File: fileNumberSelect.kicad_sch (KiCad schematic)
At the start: 13 parts, among them U17 74AHC138, U19 74AHCT244, U20 74AHCT244, U21 74AHCT244, U22 74AHCT244, U23 74AHCT244

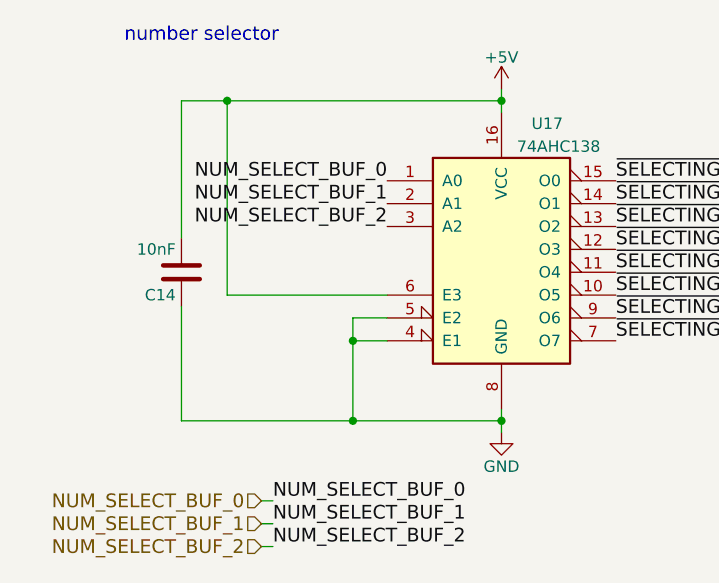
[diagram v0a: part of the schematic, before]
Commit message: bit of cleaning after last commit
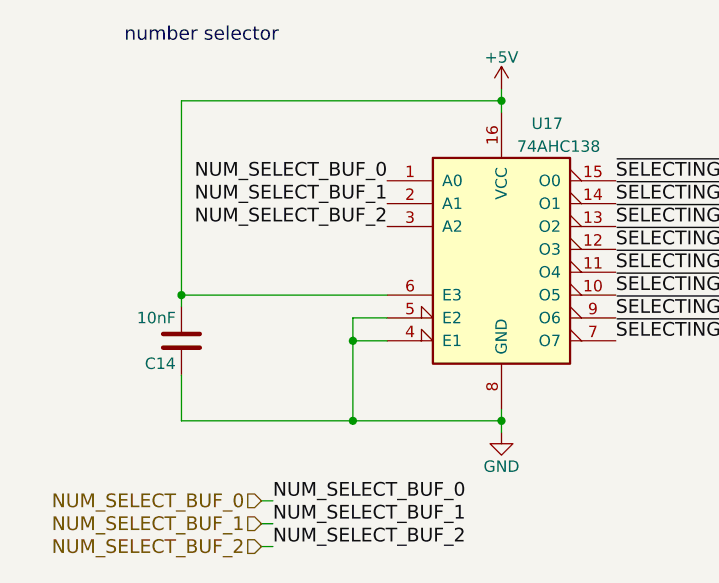
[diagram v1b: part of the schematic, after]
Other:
- moved on the sheet: C14
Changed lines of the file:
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@@
   (junction (at 62.23 24.13) (diameter 0) (color 0 0 0 0)
   )
+  (junction (at 26.67 45.72) (diameter 0) (color 0 0 0 0)
+  )
   (junction (at 238.76 149.86) (diameter 0) (color 0 0 0 0)
   )
@@
   (junction (at 220.98 22.86) (diameter 0) (color 0 0 0 0)
   )
-  (junction (at 31.75 24.13) (diameter 0) (color 0 0 0 0)
-  )
   (junction (at 218.44 25.4) (diameter 0) (color 0 0 0 0)
   )
@@
     (stroke (width 0) (type default) (color 0 0 0 0))
   )
-  (wire (pts (xy 31.75 24.13) (xy 31.75 45.72))
-    (stroke (width 0) (type default) (color 0 0 0 0))
-  )
   (wire (pts (xy 137.16 171.45) (xy 139.7 171.45))
     (stroke (width 0) (type default) (color 0 0 0 0))
@@
     (stroke (width 0) (type default) (color 0 0 0 0))
   )
-  (wire (pts (xy 31.75 24.13) (xy 26.67 24.13))
+  (wire (pts (xy 26.67 24.13) (xy 62.23 24.13))
     (stroke (width 0) (type default) (color 0 0 0 0))
   )
@@
     (stroke (width 0) (type default) (color 0 0 0 0))
   )
-  (wire (pts (xy 26.67 46.99) (xy 26.67 59.69))
+  (wire (pts (xy 26.67 54.61) (xy 26.67 59.69))
     (stroke (width 0) (type default) (color 0 0 0 0))
   )
@@
     (stroke (width 0) (type default) (color 0 0 0 0))
   )
-  (wire (pts (xy 26.67 24.13) (xy 26.67 39.37))
+  (wire (pts (xy 26.67 24.13) (xy 26.67 45.72))
     (stroke (width 0) (type default) (color 0 0 0 0))
   )
@@
     (stroke (width 0) (type default) (color 0 0 0 0))
   )
+  (wire (pts (xy 26.67 45.72) (xy 26.67 46.99))
+    (stroke (width 0) (type default) (color 0 0 0 0))
+  )
   (wire (pts (xy 43.18 151.13) (xy 44.45 151.13))
     (stroke (width 0) (type default) (color 0 0 0 0))
@@
     (stroke (width 0) (type default) (color 0 0 0 0))
   )
-  (wire (pts (xy 62.23 24.13) (xy 31.75 24.13))
-    (stroke (width 0) (type default) (color 0 0 0 0))
-  )
-  (wire (pts (xy 49.53 45.72) (xy 31.75 45.72))
+  (wire (pts (xy 26.67 45.72) (xy 49.53 45.72))
     (stroke (width 0) (type default) (color 0 0 0 0))
   )
@@
     (pin "1")
   )
-  (symbol (lib_id "Device:C") (at 26.67 43.18 180) (unit 1)
+  (symbol (lib_id "Device:C") (at 26.67 50.8 180) (unit 1)
     (in_bom yes) (on_board yes)
-    (property "Reference" "C14" (id 0) (at 26.035 45.72 0)
+    (property "Reference" "C14" (id 0) (at 26.035 53.34 0)
       (effects (font (size 1.27 1.27)) (justify left))
     )
-    (property "Value" "10nF" (id 1) (at 26.035 40.64 0)
+    (property "Value" "10nF" (id 1) (at 26.035 48.26 0)
       (effects (font (size 1.27 1.27)) (justify left))
     )
-    (property "Footprint" "Capacitor_SMD:C_0805_2012Metric" (id 2) (at 25.7048 39.37 0)
+    (property "Footprint" "Capacitor_SMD:C_0805_2012Metric" (id 2) (at 25.7048 46.99 0)
       (effects (font (size 1.27 1.27)) hide)
     )
-    (property "Datasheet" "" (id 3) (at 26.67 43.18 0)
+    (property "Datasheet" "" (id 3) (at 26.67 50.8 0)
       (effects (font (size 1.27 1.27)) hide)
     )
